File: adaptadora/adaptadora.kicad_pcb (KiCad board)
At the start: 2 copper layers, 199.4 x 99.1 mm, 105 parts, among them J1 Conn_Coaxial, J10 Conn_Coaxial, J11 Conn_Coaxial, J12 Conn_Coaxial, J13 Conn_Coaxial, J14 Conn_Coaxial, J15 Conn_Coaxial, J16 Conn_Coaxial, J17 Conn_Coaxial, J18 Conn_Coaxial, J19 Conn_Coaxial, J2 Conn_Coaxial, J20 Conn_Coaxial, J21 Conn_Coaxial, J22 Conn_Coaxial, J23 Conn_Coaxial, J3 Conn_Coaxial, J4 Conn_Coaxial, J5 Conn_02x20_Odd_Even, J6 Conn_01x02, J7 Conn_02x20_Odd_Even, J8 Conn_01x04, J9 Conn_01x02, U11 LM361MX_NOPB, U12 LM361MX_NOPB, U13 LM361MX_NOPB, U14 LM361MX_NOPB, U21 TLV2772IDR, U22 TLV2772IDR, U23 TLV2772IDR, U24 TLV2772IDR, U25 TLV2772IDR, U31 SN74LVC2T45DCUR, U32 SN74LVC2T45DCUR

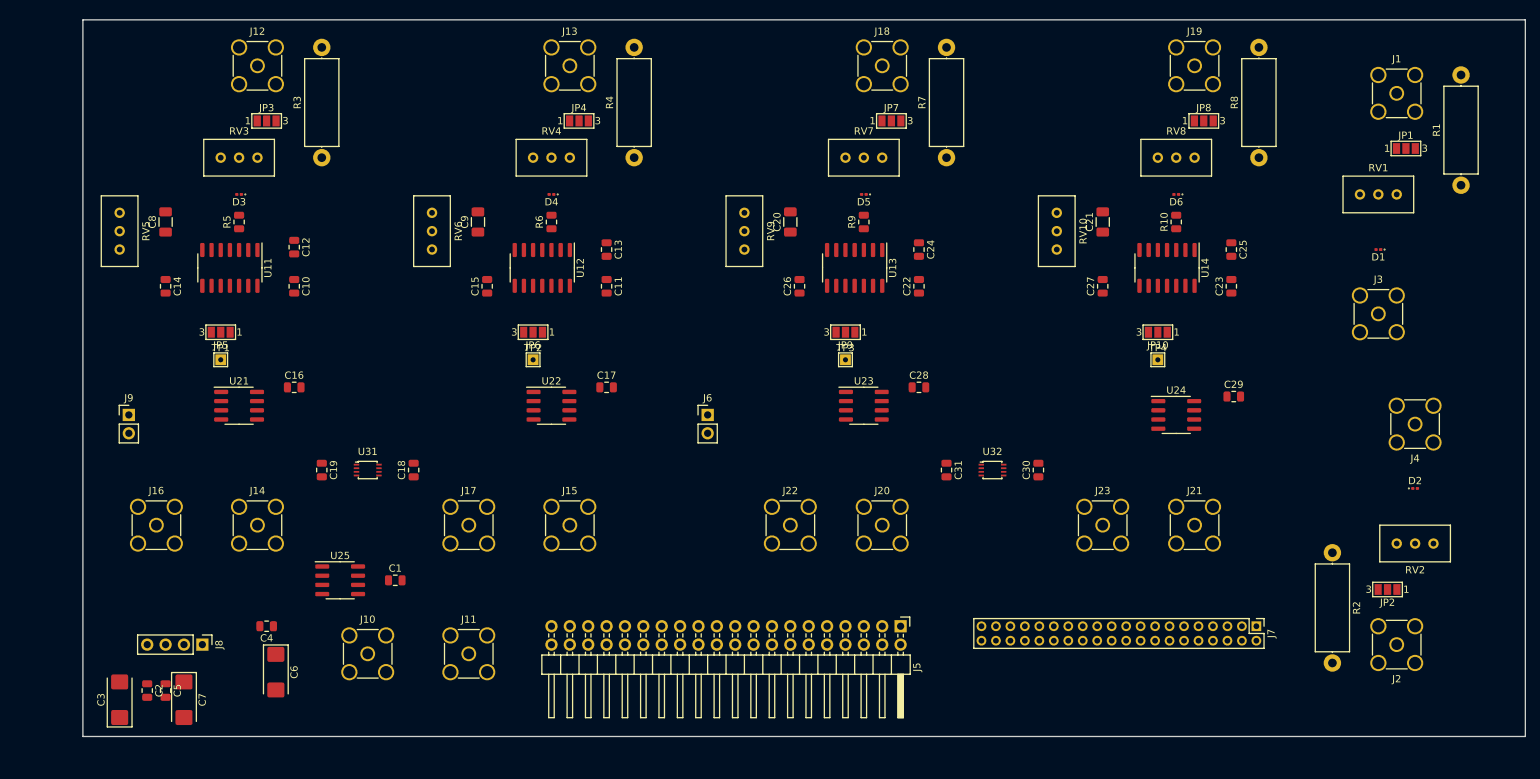
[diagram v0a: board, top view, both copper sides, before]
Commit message: pcb, work in progress
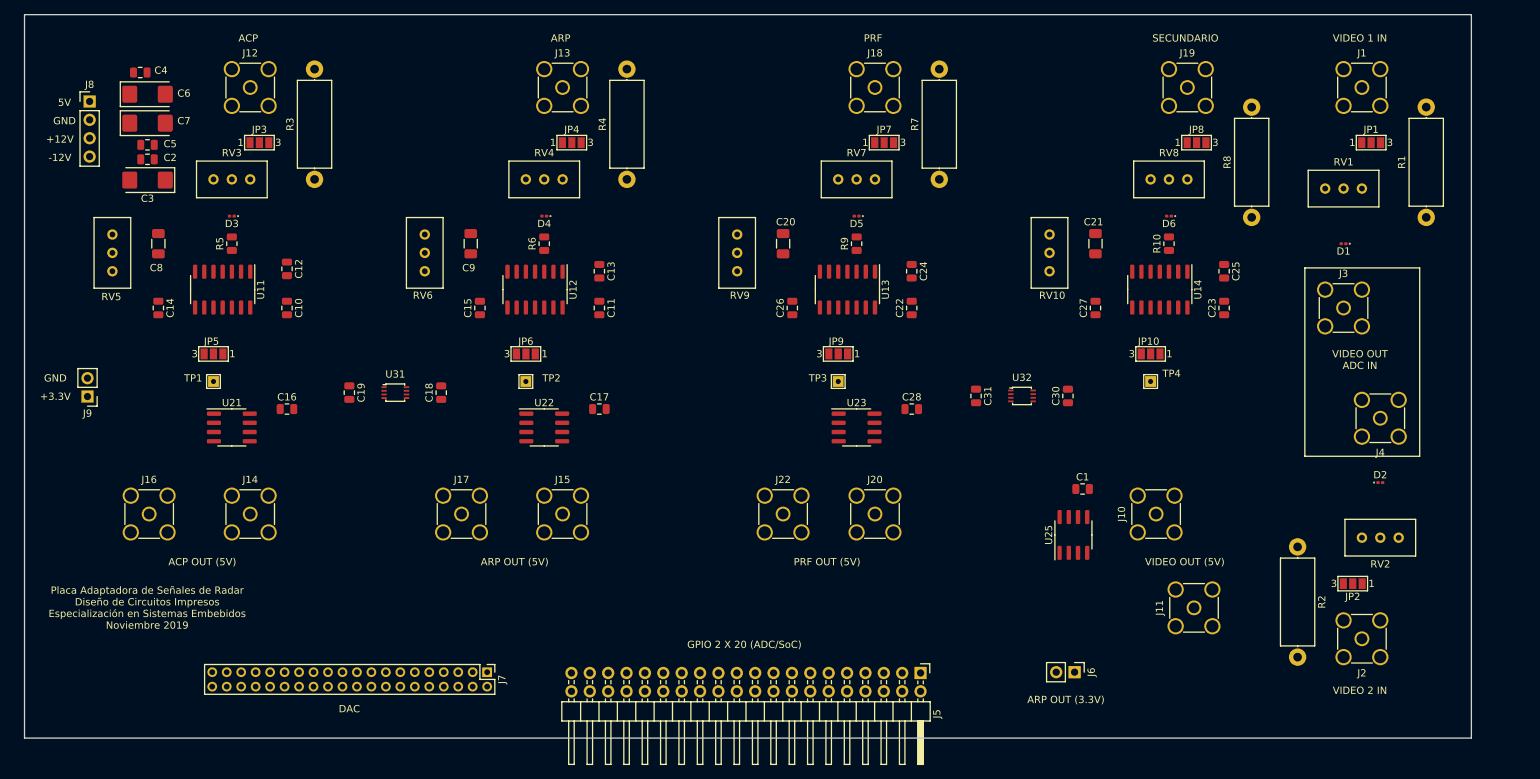
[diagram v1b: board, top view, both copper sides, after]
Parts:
- removed C29: 0.1uF-50V, Capacitor_SMD:C_0805_2012Metric
- removed J21, J23: Conn_Coaxial, Connector_Coaxial:SMA_Amphenol_901-144_Vertical
- removed U24: TLV2772IDR, Package_SO:SOIC-8_3.9x4.9mm_P1.27mm
- moved J10 110.7 mm to (200.4, 114.0), turned to 90 degrees
- moved J7 106.5 mm to (108.0, 135.9)
- moved U25 101.6 mm to (189.0, 116.9), turned to 90 degrees
- moved J11 100.5 mm to (205.7, 127.0), turned to 90 degrees
- moved C1 95.8 mm to (190.3, 110.6)
- moved C6 81.8 mm to (61.0, 56.0), turned to 0 degrees
- moved C7 79.9 mm to (61.0, 60.0), turned to 0 degrees
- moved C4 78.5 mm to (60.0, 53.0), turned to 0 degrees
- moved J8 76.7 mm to (53.0, 57.0), turned to 0 degrees
- moved C5 75.5 mm to (61.0, 63.0), turned to 0 degrees
- moved C2 73.4 mm to (61.0, 65.0), turned to 0 degrees
- moved C3 71.9 mm to (61.0, 67.9), turned to 180 degrees
- moved J6 61.9 mm to (189.2, 135.9), turned to 270 degrees
- moved C19 11.4 mm to (88.9, 97.2)
- moved U31 11.4 mm to (95.2, 97.2)
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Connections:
- C14 pad 1: -12V -> GND
- C14 pad 2: GND -> -12V
- C15 pad 1: -12V -> GND
- C15 pad 2: GND -> -12V
- C2 pad 1: -12V -> GND
- C2 pad 2: GND -> -12V
- C26 pad 1: -12V -> GND
- C26 pad 2: GND -> -12V
- C27 pad 1: -12V -> GND
- C27 pad 2: GND -> -12V
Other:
- board size 199.4 x 99.1 mm -> 200 x 100 mm
- board text added: "+12V"
- board text added: "+3.3V"
- board text added: "-12V"
- board text added: "5V"
- board text added: "ACP"
- board text added: "ACP OUT (5V)"
- board text added: "ARP"
- board text added: "ARP OUT (3.3V)"
- board text added: "ARP OUT (5V)"
- board text added: "DAC"
- board text added: "GND"
- board text added: "GPIO 2 X 20 (ADC/SoC)"
- board text added: "PRF"
- board text added: "PRF OUT (5V)"
- board text added: "Placa Adaptadora de Señales de Radar Diseño de Circuitos Impresos Especialización en Sistemas Embebidos Noviembre 2019"
- board text added: "SECUNDARIO"
- board text added: "VIDEO 1 IN"
- board text added: "VIDEO 2 IN"
- board text added: "VIDEO OUT (5V)"
- board text added: "VIDEO OUT ADC IN"
